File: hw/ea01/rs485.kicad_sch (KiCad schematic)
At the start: 15 parts, among them J6 Screw_Terminal_01x03, U12 SN75176AP

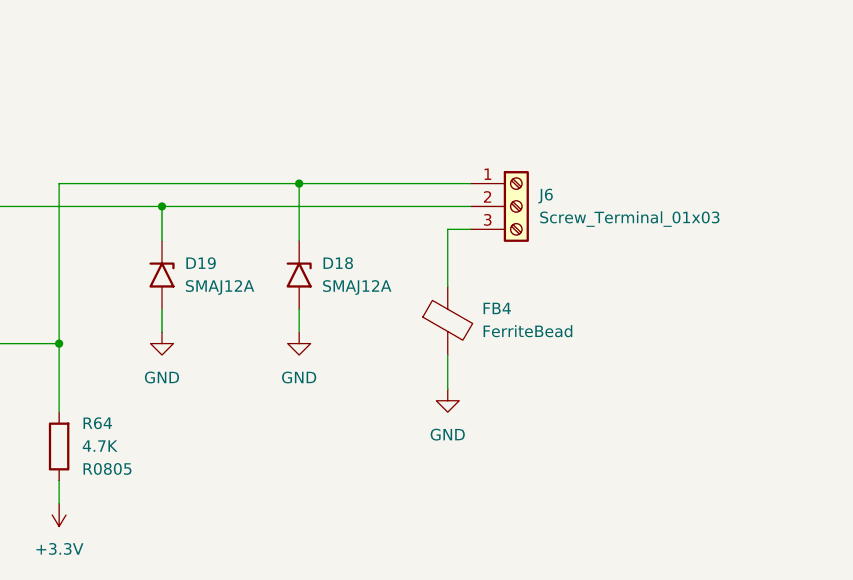
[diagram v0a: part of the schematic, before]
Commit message: draw contleted. Not checked yet.
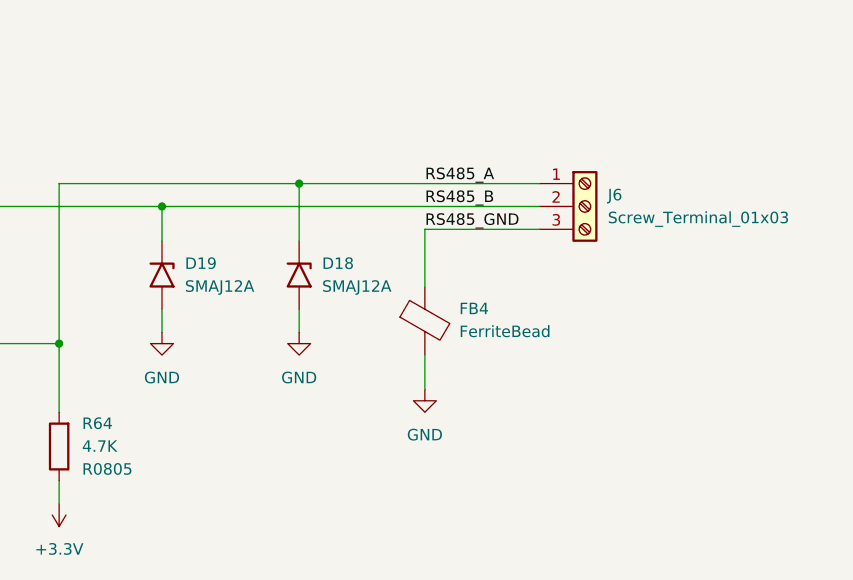
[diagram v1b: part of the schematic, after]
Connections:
- net RS485_A: now reaches D18.1 (A1), J6.1 (Pin_1), R62.1, R64.2
- net RS485_B: now reaches D19.1 (A1), J6.2 (Pin_2), R61.2, R63.2
- net RS485_GND: now reaches FB4.1, J6.3 (Pin_3)
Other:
- moved on the sheet: FB4, J6
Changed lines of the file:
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@@
+	(wire
+		(pts
+			(xy 217.17 87.63) (xy 217.17 93.98)
+		)
+		(stroke
+			(width 0)
+			(type default)
+		)
+	)
 	(wire
 		(pts
@@
 	(wire
 		(pts
-			(xy 187.96 85.09) (xy 222.25 85.09)
+			(xy 187.96 85.09) (xy 229.87 85.09)
 		)
 		(stroke
@@
 	(wire
 		(pts
-			(xy 203.2 82.55) (xy 222.25 82.55)
+			(xy 203.2 82.55) (xy 229.87 82.55)
 		)
 		(stroke
@@
 	(wire
 		(pts
-			(xy 219.71 87.63) (xy 222.25 87.63)
-		)
-		(stroke
-			(width 0)
-			(type default)
-		)
-	)
-	(wire
-		(pts
 			(xy 83.82 86.36) (xy 86.36 86.36)
 		)
@@
 	(wire
 		(pts
+			(xy 229.87 87.63) (xy 217.17 87.63)
+		)
+		(stroke
+			(width 0)
+			(type default)
+		)
+	)
+	(wire
+		(pts
 			(xy 99.06 68.58) (xy 99.06 71.12)
 		)
@@
 	(wire
 		(pts
-			(xy 219.71 101.6) (xy 219.71 105.41)
-		)
-		(stroke
-			(width 0)
-			(type default)
-		)
-	)
-	(wire
-		(pts
-			(xy 219.71 93.98) (xy 219.71 87.63)
+			(xy 217.17 101.6) (xy 217.17 105.41)
 		)
 		(stroke
@@
 			(width 0)
 			(type default)
+		)
+	)
+	(label "RS485_GND"
+		(at 217.17 87.63 0)
+		(effects
+			(font
+				(size 1.27 1.27)
+			)
+			(justify left bottom)
+		)
+	)
+	(label "RS485_B"
+		(at 217.17 85.09 0)
+		(effects
+			(font
+				(size 1.27 1.27)
+			)
+			(justify left bottom)
+		)
+	)
+	(label "RS485_A"
+		(at 217.17 82.55 0)
+		(effects
+			(font
+				(size 1.27 1.27)
+			)
+			(justify left bottom)
 		)
 	)
@@
 	(symbol
 		(lib_id "Connector:Screw_Terminal_01x03")
-		(at 227.33 85.09 0)
+		(at 234.95 85.09 0)
 		(unit 1)
 		(exclude_from_sim no)
@@
 		(fields_autoplaced yes)
 		(property "Reference" "J6"
-			(at 229.87 83.8199 0)
+			(at 237.49 83.8199 0)
 			(effects
 				(font
@@
 		)
 		(property "Value" "Screw_Terminal_01x03"
-			(at 229.87 86.3599 0)
+			(at 237.49 86.3599 0)
 			(effects
 				(font
@@
 		)
 		(property "Footprint" "TerminalBlock:TerminalBlock_bornier-3_P5.08mm"
-			(at 227.33 85.09 0)
+			(at 234.95 85.09 0)
 			(effects
 				(font
@@
 		)
 		(property "Datasheet" "~"
-			(at 227.33 85.09 0)
+			(at 234.95 85.09 0)
 			(effects
 				(font
@@
 		)
 		(property "Description" "Generic screw terminal, single row, 01x03, script generated (kicad-library-utils/schlib/autogen/connector/)"
-			(at 227.33 85.09 0)
+			(at 234.95 85.09 0)
 			(effects
 				(font
@@
 	(symbol
 		(lib_id "power:GND")
-		(at 219.71 105.41 0)
+		(at 217.17 105.41 0)
 		(unit 1)
 		(exclude_from_sim no)
@@
 		(fields_autoplaced yes)
 		(property "Reference" "#PWR0147"
-			(at 219.71 111.76 0)
+			(at 217.17 111.76 0)
 			(effects
 				(font
@@
 		)
 		(property "Value" "GND"
-			(at 219.71 110.49 0)
+			(at 217.17 110.49 0)
 			(effects
 				(font
@@
 		)
 		(property "Footprint" ""
-			(at 219.71 105.41 0)
+			(at 217.17 105.41 0)
 			(effects
 				(font
@@
 		)
 		(property "Datasheet" ""
-			(at 219.71 105.41 0)
+			(at 217.17 105.41 0)
 			(effects
 				(font
@@
 		)
 		(property "Description" "Power symbol creates a global label with name \"GND\" , ground"
-			(at 219.71 105.41 0)
+			(at 217.17 105.41 0)
 			(effects
 				(font
@@
 	(symbol
 		(lib_id "Device:FerriteBead")
-		(at 219.71 97.79 0)
+		(at 217.17 97.79 0)
 		(unit 1)
 		(exclude_from_sim no)
@@
 		(fields_autoplaced yes)
 		(property "Reference" "FB4"
-			(at 223.52 96.4691 0)
+			(at 220.98 96.4691 0)
 			(effects
 				(font
@@
 		)
 		(property "Value" "FerriteBead"
-			(at 223.52 99.0091 0)
+			(at 220.98 99.0091 0)
 			(effects
 				(font
@@
 		)
 		(property "Footprint" "Resistor_SMD:R_0805_2012Metric"
-			(at 217.932 97.79 90)
+			(at 215.392 97.79 90)
 			(effects
 				(font
@@
 		)
 		(property "Datasheet" "~"
-			(at 219.71 97.79 0)
+			(at 217.17 97.79 0)
 			(effects
 				(font
@@
 		)
 		(property "Description" "Ferrite bead"
-			(at 219.71 97.79 0)
-			(effects
-				(font
+			(at 217.17 97.79 0)
+			(effects
+				(font
